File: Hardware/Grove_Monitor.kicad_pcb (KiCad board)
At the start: 2 copper layers, 103 x 77 mm, 81 parts, among them J1 AUDIO_JACK_3.5MM_SMD, J2 AUDIO_JACK_3.5MM_SMD, J3 QWIIC, J4 QWIIC, J5 Conn_01x03, J6 Conn_01x05, J7 Conn_01x03, J8 Conn_01x02, P1 BNC, P2 BNC, P3 BNC, P401 BNC, U1 PARTICLE_MESH, U2 ADM3260, U3 ADM3260, U4 ADM3260

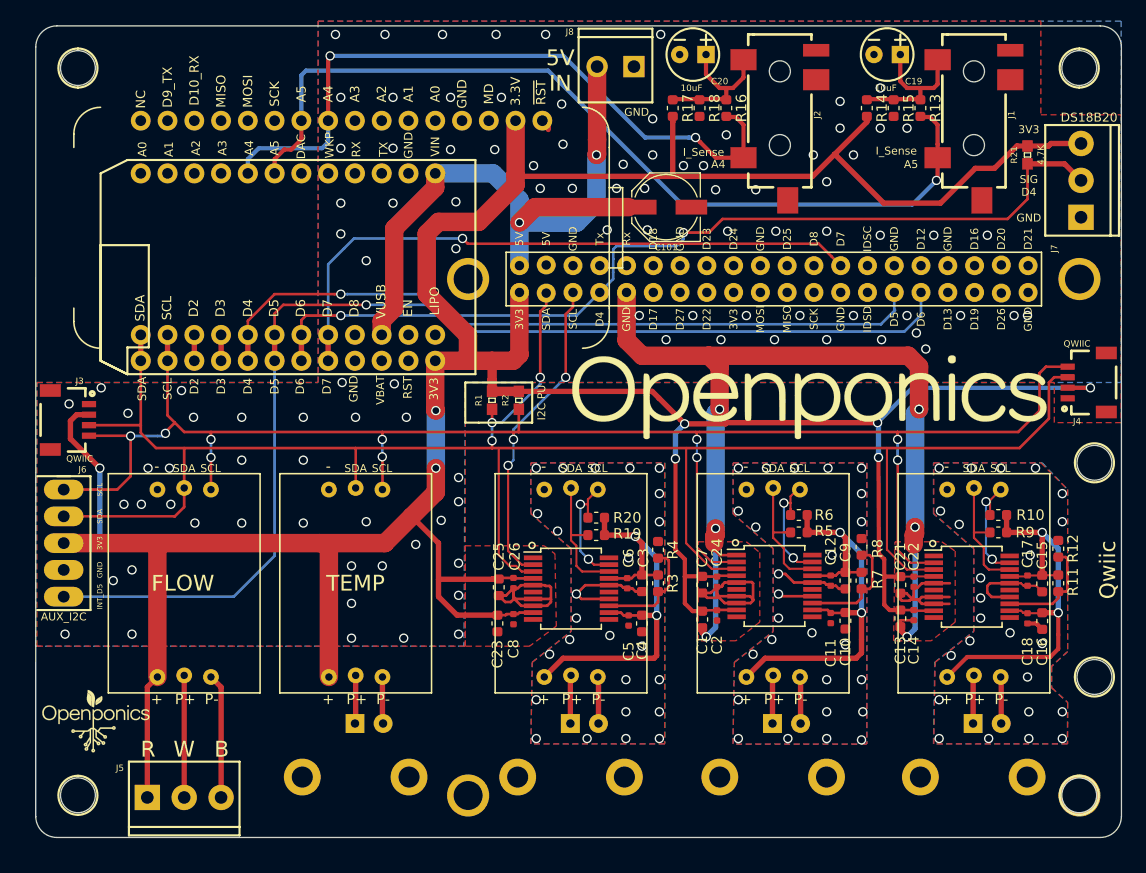
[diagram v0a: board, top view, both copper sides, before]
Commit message: V1.0 Complete
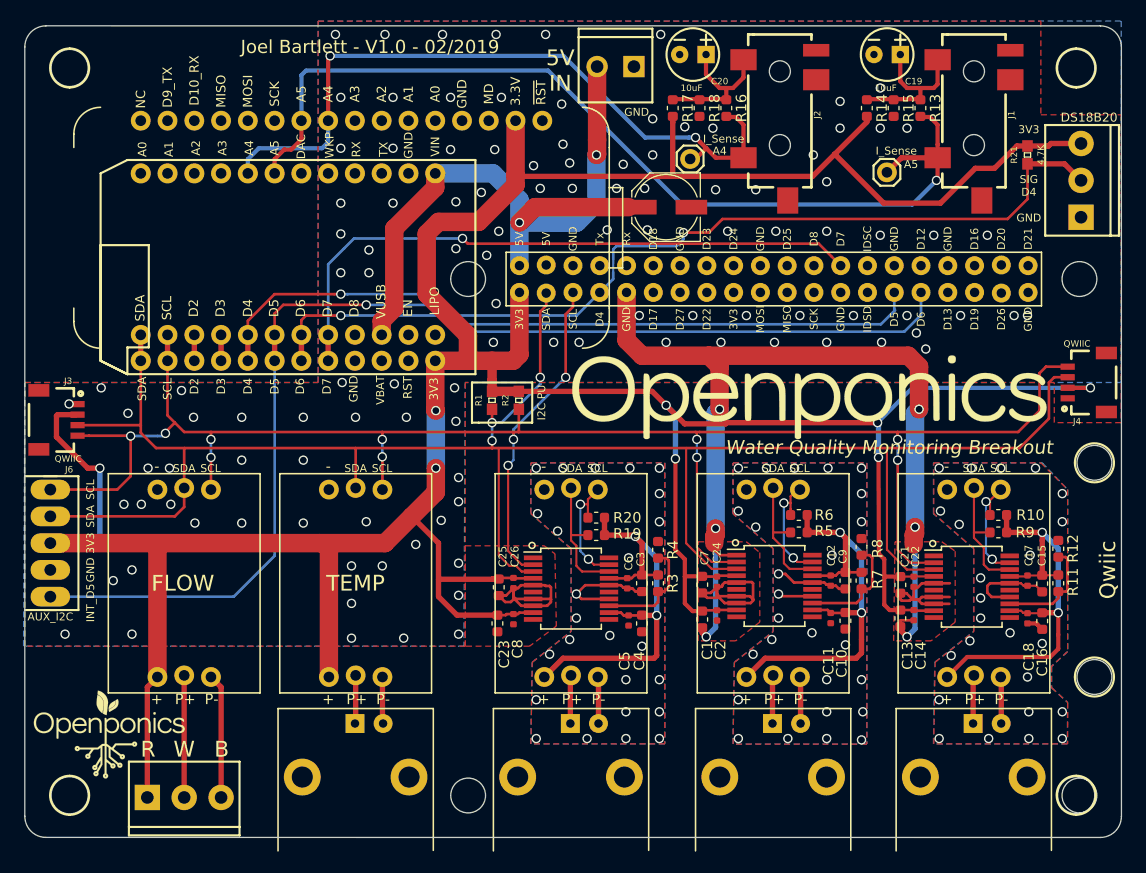
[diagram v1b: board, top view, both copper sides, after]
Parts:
- added J10: Conn_01x01, Connectors:1X01, F.Cu at (119.1, 95.6)
- added J9: Conn_01x01, Connectors:1X01, F.Cu at (137.8, 96.9)
- H1, H2, H3, H4: footprint MeowWolf_Hardware:STAND-OFF -> Openponics_Hardware:STAND-OFF_LARGE
- LOGO2: footprint Openponics_Logos:Openponics_Logo_Horizontal_10mm -> Openponics_Logos:Openponics_Logo_Horizontal_16mm
- PI_Board: footprint temp_terminal:WL-PI_Board_no_outline -> Openponics_Hardware:RAS_PI_MOUNTING_HOLES
- moved LOGO2 1.80 mm to (64.0, 150.2)
- moved J6 1.27 mm to (58.4, 137.2)
- moved J3 1.09 mm to (61.0, 120.4)
- moved H1 0.79 mm to (60.2, 87.0)
- moved H2 0.79 mm to (60.2, 156.0)
- moved H3 0.29 mm to (155.8, 156.0)
- moved H4 0.29 mm to (155.8, 87.0)
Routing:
- net A5: track 84.7 -> 90.1 mm
- net +3V3: track 366.0 -> 369.5 mm
- net SDA: track 191.1 -> 193.8 mm
- net SCL: track 192.1 -> 194.8 mm
- net A4: track 66.2 -> 68.1 mm
- net (no net): track 1.07 -> 0.00 mm
- net GND: vias 111 -> 121
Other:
- board size 103 x 77 mm -> 104 x 77 mm
- board text added: "Joel Bartlett - V1.0 - 02/2019"
- board text added: "Water Quality Monitoring Breakout"
- board text removed: "STP (2/2)"
